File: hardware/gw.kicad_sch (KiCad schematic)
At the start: 21 parts, among them J1 USB_OTG, J2 Conn_01x04, U1 ESP-12F, U2 Ai-Thinker-Ra-02, U3 AMS1117-3.3

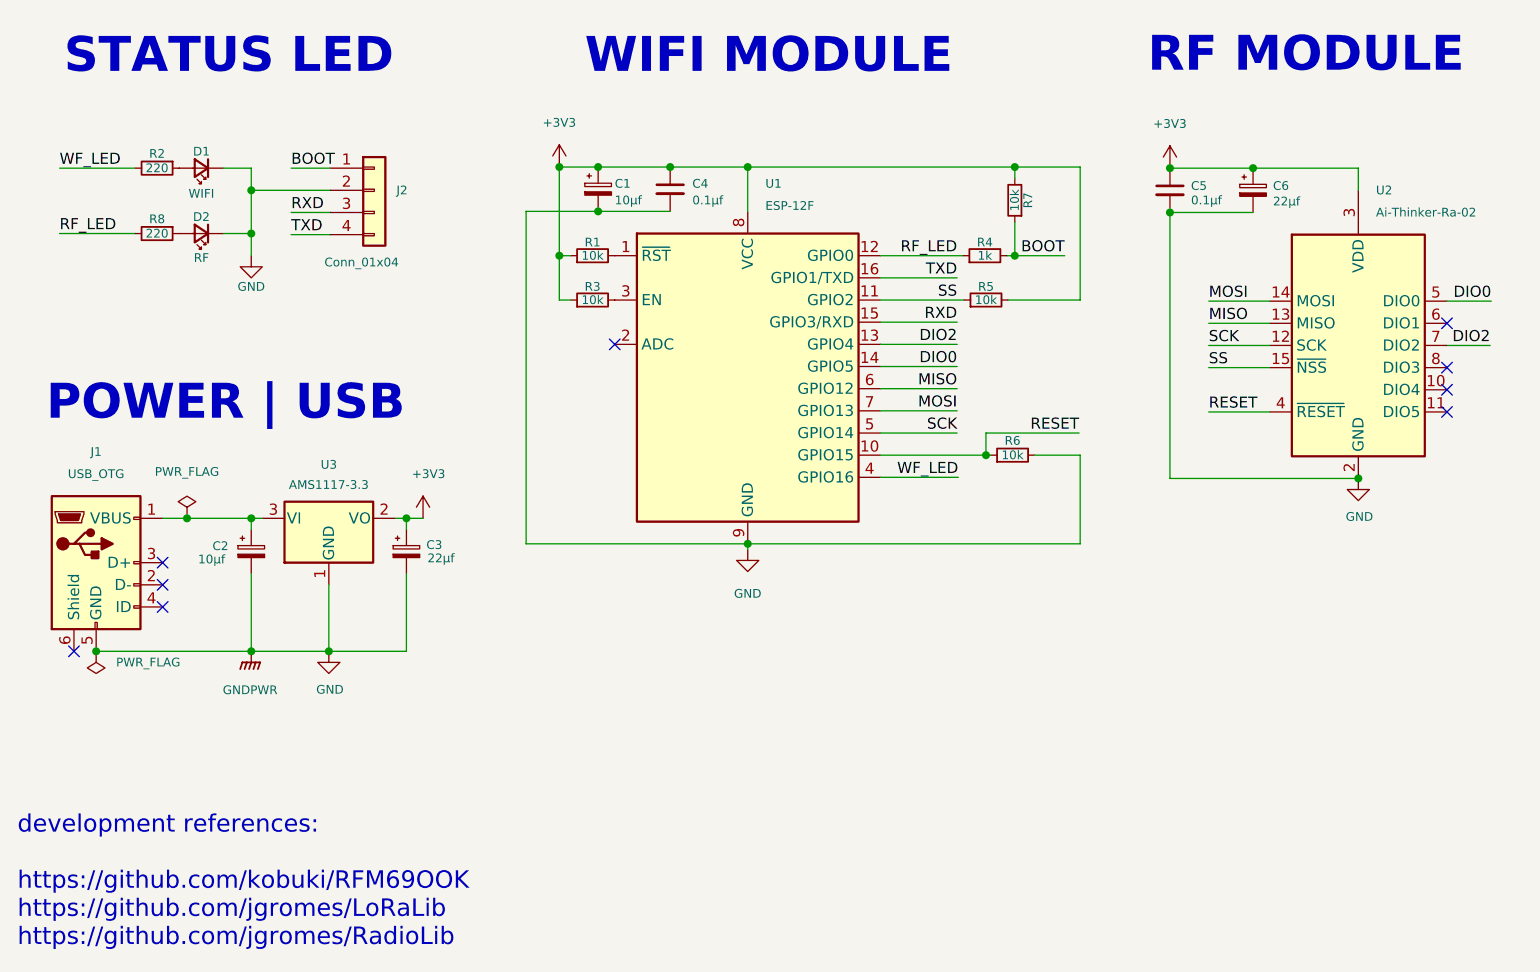
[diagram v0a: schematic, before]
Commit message: Fixes
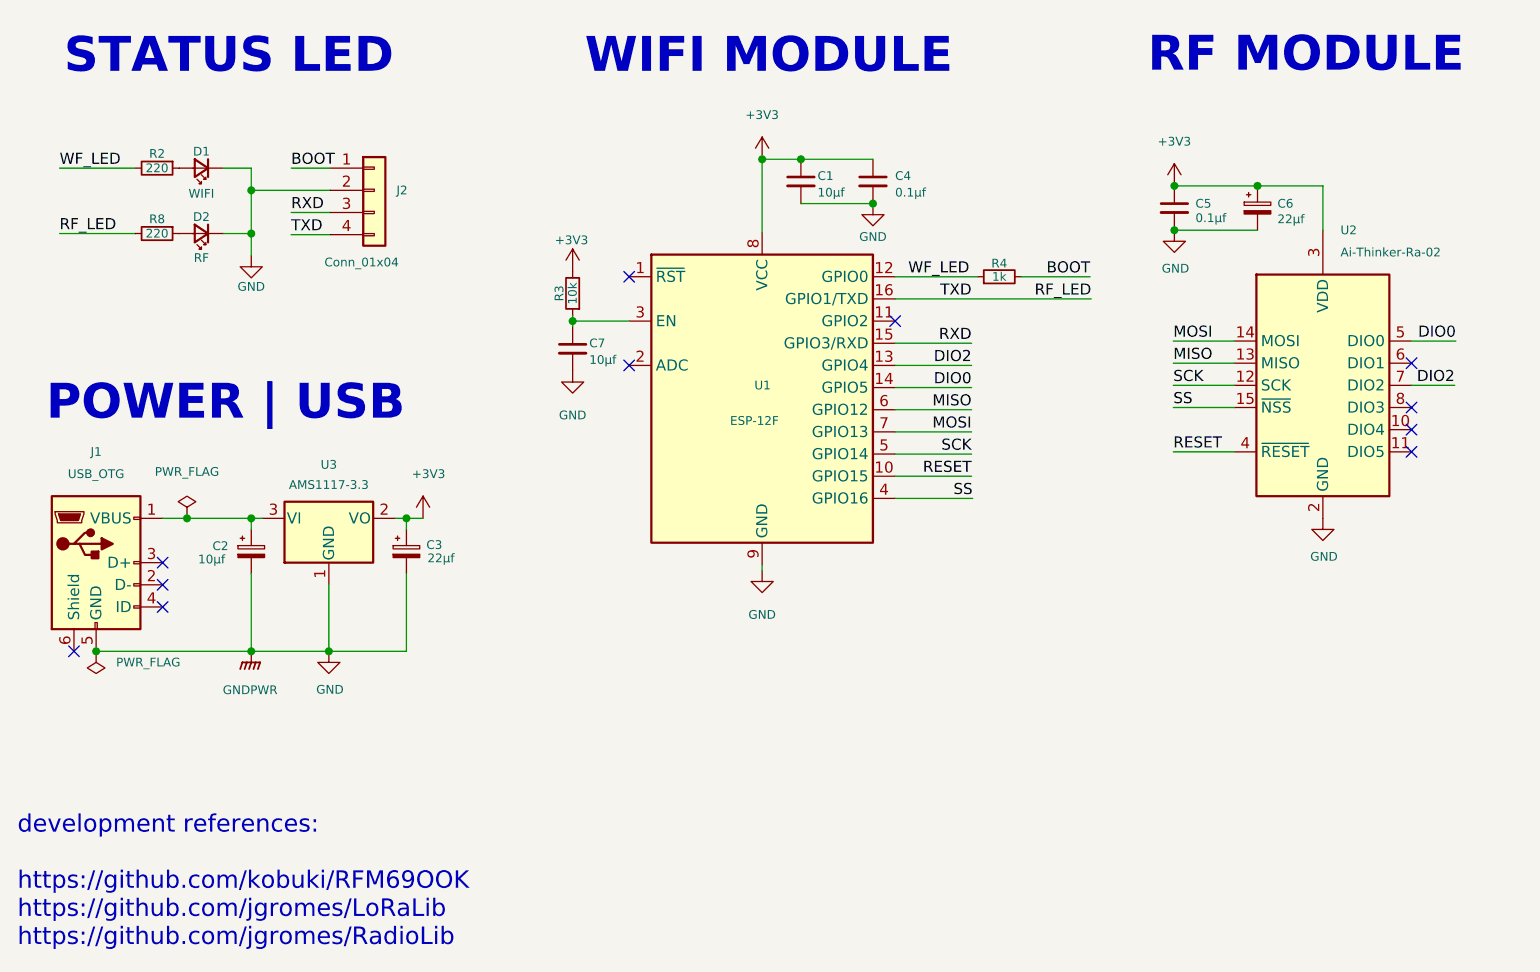
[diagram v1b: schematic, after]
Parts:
- removed R1, R5, R6, R7: 10k, Resistor_SMD:R_1206_3216Metric, symbol Device:R_Small
- added C7: 10µf, Capacitor_SMD:C_1206_3216Metric, symbol Device:C_Small
- C1: footprint Capacitor_Tantalum_SMD:CP_EIA-3216-10_Kemet-I -> Capacitor_SMD:C_1206_3216Metric; symbol Device:C_Polarized_Small -> Device:C_Small
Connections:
- net TXD is gone; now on net RF_LED: J2.4 (Pin_4), U1.16 (GPIO1/TXD)
- net +3V3: now also R3.2; no longer R3.1
- net GND: now also C7.2
- net RF_LED: no longer R4.1, U1.12 (GPIO0)
- net SS: now also U1.4 (GPIO16); no longer U1.11 (GPIO2)
- net WF_LED: now also R4.1, U1.12 (GPIO0); no longer U1.4 (GPIO16)
- net at U1.3 (EN): now also R3.1, C7.1; no longer R3.2
- no-connect marks 9 -> 11
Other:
- moved on the sheet: C4, C5, C6, R3, R4, U1, U2
